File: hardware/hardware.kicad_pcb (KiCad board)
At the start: 2 copper layers, 14 parts, among them U1 ESP32-DEVKITC-32D

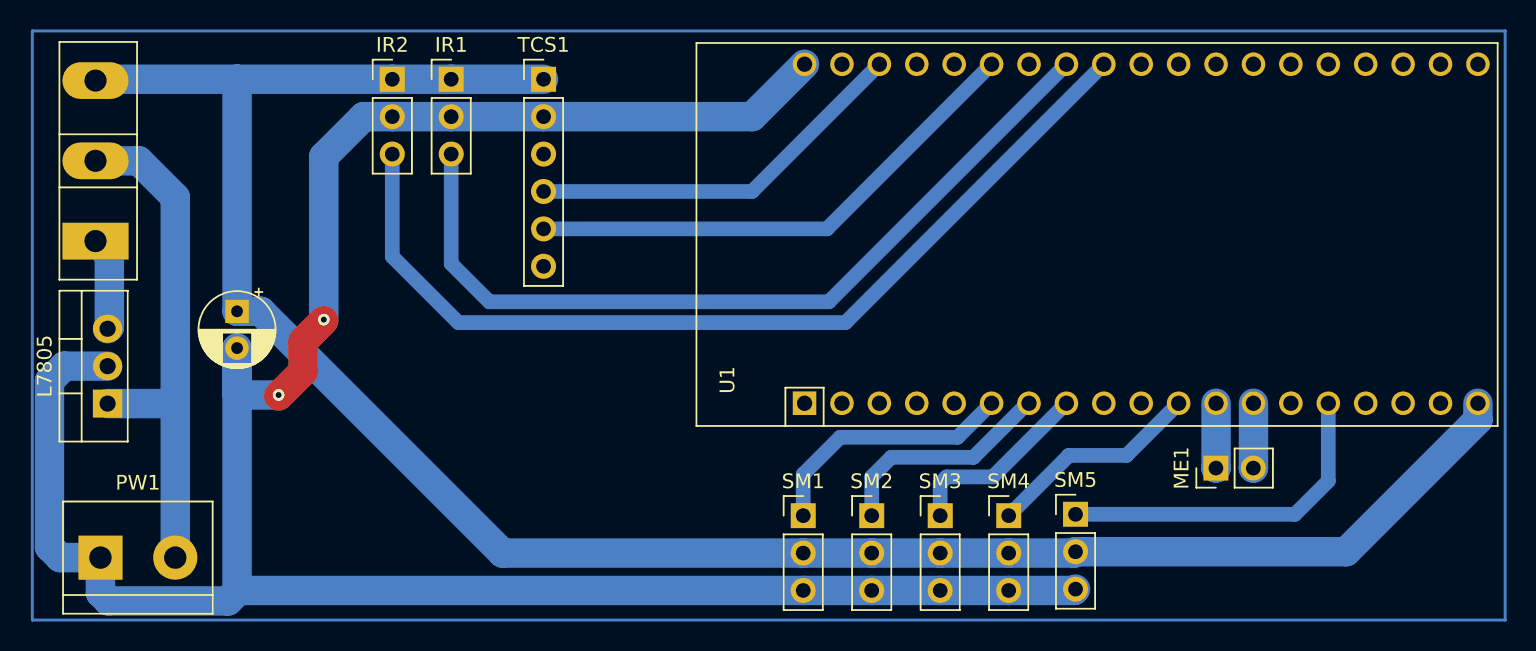
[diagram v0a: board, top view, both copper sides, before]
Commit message: fix: login
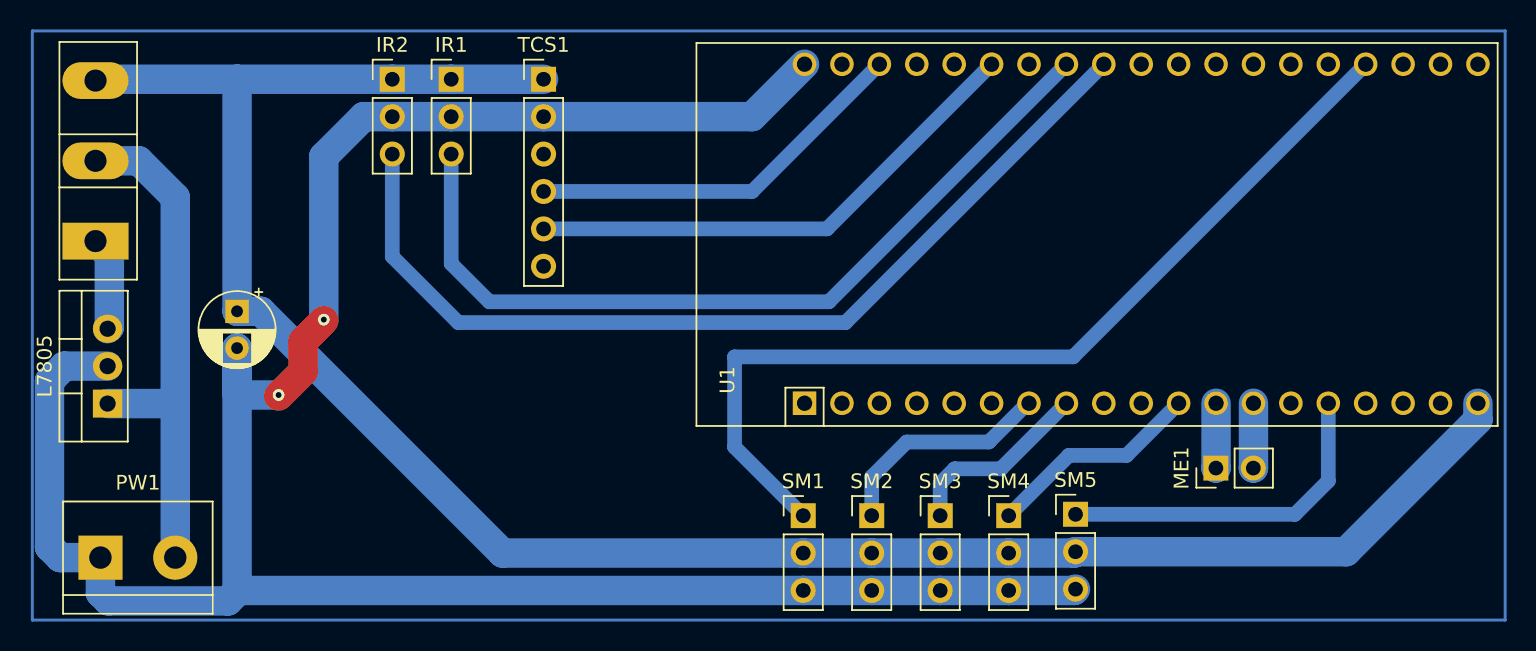
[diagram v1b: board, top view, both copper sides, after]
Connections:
- U1 pad 35: (no net) -> Net-(SM1-Pin_1)
- U1 pad 6: Net-(SM1-Pin_1) -> (no net)
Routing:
- net Net-(SM1-Pin_1): track 17.6 -> 63.8 mm
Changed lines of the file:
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@@
     (pad "4" thru_hole circle (at 0.241 7.62 90) (size 1.6 1.6) (drill 1.04) (layers "*.Cu" "*.Mask"))
     (pad "5" thru_hole circle (at 0.241 10.16 90) (size 1.6 1.6) (drill 1.04) (layers "*.Cu" "*.Mask"))
-    (pad "6" thru_hole circle (at 0.241 12.7 90) (size 1.6 1.6) (drill 1.04) (layers "*.Cu" "*.Mask")
-      (net 5 "Net-(SM1-Pin_1)"))
+    (pad "6" thru_hole circle (at 0.241 12.7 90) (size 1.6 1.6) (drill 1.04) (layers "*.Cu" "*.Mask"))
     (pad "7" thru_hole circle (at 0.241 15.24 90) (size 1.6 1.6) (drill 1.04) (layers "*.Cu" "*.Mask")
       (net 6 "Net-(SM2-Pin_1)"))
@@
     (pad "33" thru_hole circle (at 23.26 33.02 90) (size 1.6 1.6) (drill 1.04) (layers "*.Cu" "*.Mask"))
     (pad "34" thru_hole circle (at 23.26 35.56 90) (size 1.6 1.6) (drill 1.04) (layers "*.Cu" "*.Mask"))
-    (pad "35" thru_hole circle (at 23.26 38.1 90) (size 1.6 1.6) (drill 1.04) (layers "*.Cu" "*.Mask"))
+    (pad "35" thru_hole circle (at 23.26 38.1 90) (size 1.6 1.6) (drill 1.04) (layers "*.Cu" "*.Mask")
+      (net 5 "Net-(SM1-Pin_1)"))
     (pad "36" thru_hole circle (at 23.26 40.64 90) (size 1.6 1.6) (drill 1.04) (layers "*.Cu" "*.Mask"))
     (pad "37" thru_hole circle (at 23.26 43.18 90) (size 1.6 1.6) (drill 1.04) (layers "*.Cu" "*.Mask"))
@@
   (segment (start 158.94 94.39) (end 158.94 99.28) (width 2) (layer "B.Cu") (net 4))
   (segment (start 158.94 99.28) (end 158.82 99.4) (width 2) (layer "B.Cu") (net 4))
-  (segment (start 216.5295 106.77) (end 208.56 106.77) (width 1) (layer "B.Cu") (net 5))
-  (segment (start 218.84 104.4595) (end 216.5295 106.77) (width 1) (layer "B.Cu") (net 5))
-  (segment (start 208.56 106.77) (end 206.05 109.28) (width 1) (layer "B.Cu") (net 5))
-  (segment (start 206.05 109.28) (end 206.05 112.09) (width 1) (layer "B.Cu") (net 5))
-  (segment (start 221.283444 104.4595) (end 217.612944 108.13) (width 1) (layer "B.Cu") (net 6))
-  (segment (start 212.0295 108.13) (end 210.7 109.4595) (width 1) (layer "B.Cu") (net 6))
+  (segment (start 224.3705 101.31) (end 201.39 101.31) (width 1) (layer "B.Cu") (net 5))
+  (segment (start 201.39 107.43) (end 206.05 112.09) (width 1) (layer "B.Cu") (net 5))
+  (segment (start 201.39 101.31) (end 201.39 107.43) (width 1) (layer "B.Cu") (net 5))
+  (segment (start 244.24 81.4405) (end 224.3705 101.31) (width 1) (layer "B.Cu") (net 5))
+  (segment (start 221.38 104.4595) (end 221.283444 104.4595) (width 1) (layer "B.Cu") (net 6))
   (segment (start 210.7 109.4595) (end 210.7 112.09) (width 1) (layer "B.Cu") (net 6))
-  (segment (start 217.612944 108.13) (end 212.0295 108.13) (width 1) (layer "B.Cu") (net 6))
-  (segment (start 221.38 104.4595) (end 221.283444 104.4595) (width 1) (layer "B.Cu") (net 6))
-  (segment (start 215.78 109.46) (end 215.35 109.89) (width 1) (layer "B.Cu") (net 7))
+  (segment (start 213.0695 107.09) (end 210.7 109.4595) (width 1) (layer "B.Cu") (net 6))
+  (segment (start 221.283444 104.4595) (end 218.652944 107.09) (width 1) (layer "B.Cu") (net 6))
+  (segment (start 218.652944 107.09) (end 213.0695 107.09) (width 1) (layer "B.Cu") (net 6))
+  (segment (start 223.92 104.4595) (end 219.4695 108.91) (width 1) (layer "B.Cu") (net 7))
   (segment (start 215.35 109.89) (end 215.35 112.09) (width 1) (layer "B.Cu") (net 7))
-  (segment (start 218.9195 109.46) (end 215.78 109.46) (width 1) (layer "B.Cu") (net 7))
-  (segment (start 223.92 104.4595) (end 218.9195 109.46) (width 1) (layer "B.Cu") (net 7))
+  (segment (start 216.33 108.91) (end 215.35 109.89) (width 1) (layer "B.Cu") (net 7))
+  (segment (start 219.4695 108.91) (end 216.33 108.91) (width 1) (layer "B.Cu") (net 7))
   (segment (start 231.54 104.4595) (end 227.9995 108) (width 1) (layer "B.Cu") (net 8))
   (segment (start 227.9995 108) (end 224.09 108) (width 1) (layer "B.Cu") (net 8))
